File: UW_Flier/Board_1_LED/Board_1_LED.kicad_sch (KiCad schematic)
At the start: 11 parts, among them J1 RESET, J2 SWDIO, J3 SWDCLK, J4 GND, J5 VDD, J6 LED_DRAIN, Q1 CSD13385F5, U1 EYSHSNZWZ_module_stub

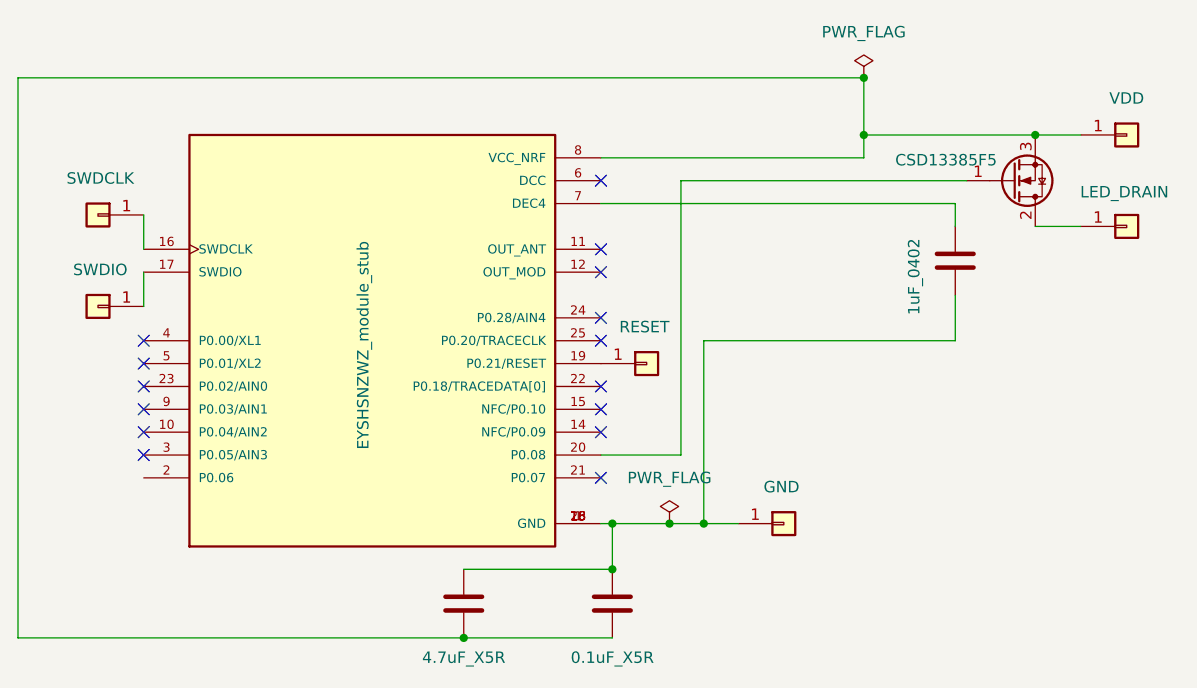
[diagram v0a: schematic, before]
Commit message: stuff
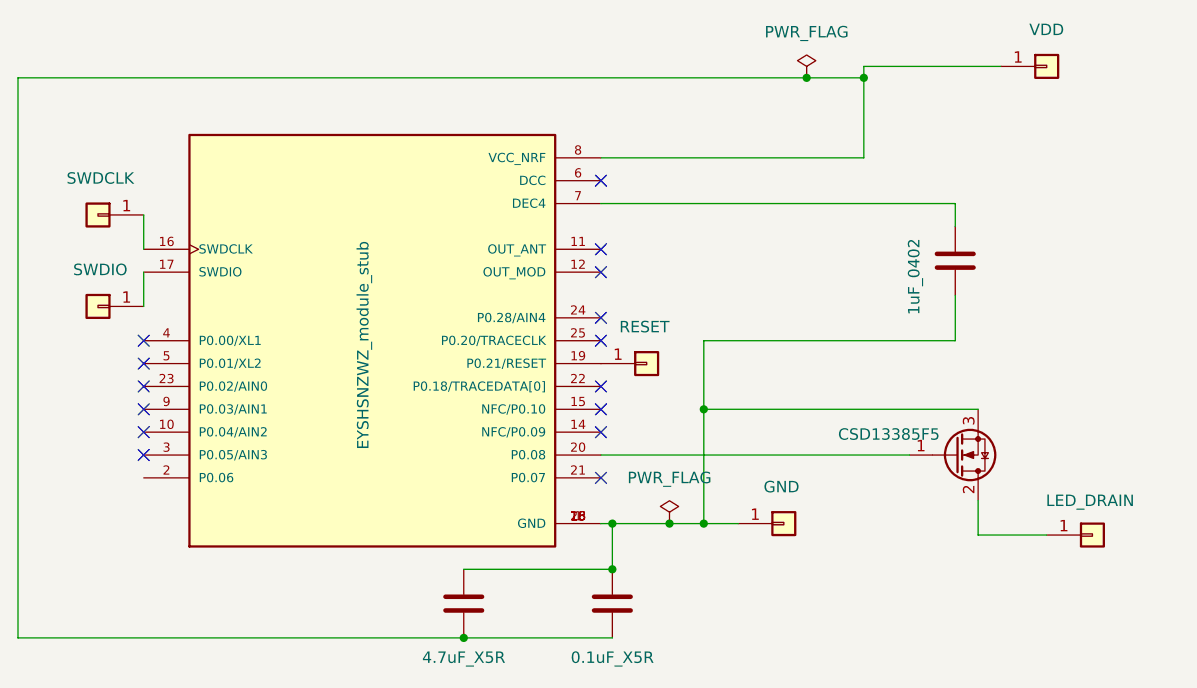
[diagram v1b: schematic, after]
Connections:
- net at C1.2, C2.2, C3.2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: now also Q1.3 (S)
- net at C1.1, C2.1, J5.1 (Pin_1)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: no longer Q1.3 (S)
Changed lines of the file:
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@@
+	)
+	(junction
+		(at 119.38 43.18)
+		(diameter 0)
+		(color 0 0 0 0)
 	)
 	(junction
@@
 	)
 	(junction
-		(at 144.78 49.53)
-		(diameter 0)
-		(color 0 0 0 0)
-	)
-	(junction
 		(at 107.95 92.71)
-		(diameter 0)
-		(color 0 0 0 0)
-	)
-	(junction
-		(at 125.73 49.53)
 		(diameter 0)
 		(color 0 0 0 0)
@@
 	)
 	(junction
+		(at 107.95 80.01)
+		(diameter 0)
+		(color 0 0 0 0)
+	)
+	(junction
 		(at 97.79 97.79)
 		(diameter 0)
@@
 	(wire
 		(pts
-			(xy 125.73 43.18) (xy 125.73 49.53)
+			(xy 125.73 43.18) (xy 125.73 52.07)
 		)
 		(stroke
@@
 	(wire
 		(pts
+			(xy 140.97 41.91) (xy 125.73 41.91)
+		)
+		(stroke
+			(width 0)
+			(type default)
+		)
+	)
+	(wire
+		(pts
 			(xy 31.75 105.41) (xy 31.75 43.18)
 		)
@@
 	(wire
 		(pts
-			(xy 144.78 59.69) (xy 149.86 59.69)
-		)
-		(stroke
-			(width 0)
-			(type default)
-		)
-	)
-	(wire
-		(pts
 			(xy 135.89 67.31) (xy 135.89 72.39)
 		)
@@
 	(wire
 		(pts
+			(xy 125.73 41.91) (xy 125.73 43.18)
+		)
+		(stroke
+			(width 0)
+			(type default)
+		)
+	)
+	(wire
+		(pts
 			(xy 97.79 92.71) (xy 104.14 92.71)
 		)
@@
 	(wire
 		(pts
-			(xy 125.73 49.53) (xy 144.78 49.53)
+			(xy 138.43 93.98) (xy 138.43 90.17)
+		)
+		(stroke
+			(width 0)
+			(type default)
+		)
+	)
+	(wire
+		(pts
+			(xy 107.95 80.01) (xy 138.43 80.01)
+		)
+		(stroke
+			(width 0)
+			(type default)
+		)
+	)
+	(wire
+		(pts
+			(xy 107.95 80.01) (xy 107.95 92.71)
 		)
 		(stroke
@@
 	(wire
 		(pts
-			(xy 144.78 49.53) (xy 149.86 49.53)
-		)
-		(stroke
-			(width 0)
-			(type default)
-		)
-	)
-	(wire
-		(pts
 			(xy 96.52 52.07) (xy 125.73 52.07)
 		)
@@
 	(wire
 		(pts
+			(xy 146.05 93.98) (xy 138.43 93.98)
+		)
+		(stroke
+			(width 0)
+			(type default)
+		)
+	)
+	(wire
+		(pts
+			(xy 119.38 43.18) (xy 125.73 43.18)
+		)
+		(stroke
+			(width 0)
+			(type default)
+		)
+	)
+	(wire
+		(pts
 			(xy 97.79 92.71) (xy 97.79 97.79)
 		)
@@
 	(wire
 		(pts
-			(xy 107.95 72.39) (xy 107.95 92.71)
+			(xy 107.95 72.39) (xy 107.95 80.01)
 		)
 		(stroke
@@
 	(wire
 		(pts
-			(xy 96.52 85.09) (xy 105.41 85.09)
+			(xy 96.52 85.09) (xy 130.81 85.09)
 		)
 		(stroke
@@
 	(wire
 		(pts
-			(xy 31.75 43.18) (xy 125.73 43.18)
-		)
-		(stroke
-			(width 0)
-			(type default)
-		)
-	)
-	(wire
-		(pts
-			(xy 105.41 54.61) (xy 137.16 54.61)
+			(xy 31.75 43.18) (xy 119.38 43.18)
 		)
 		(stroke
@@
 		(pts
 			(xy 135.89 57.15) (xy 135.89 59.69)
-		)
-		(stroke
-			(width 0)
-			(type default)
-		)
-	)
-	(wire
-		(pts
-			(xy 125.73 52.07) (xy 125.73 49.53)
-		)
-		(stroke
-			(width 0)
-			(type default)
-		)
-	)
-	(wire
-		(pts
-			(xy 105.41 54.61) (xy 105.41 85.09)
 		)
 		(stroke
@@
 	(symbol
 		(lib_id "power:PWR_FLAG")
-		(at 125.73 43.18 0)
+		(at 119.38 43.18 0)
 		(unit 1)
 		(exclude_from_sim no)
@@
 		(fields_autoplaced yes)
 		(property "Reference" "#FLG01"
-			(at 125.73 41.275 0)
+			(at 119.38 41.275 0)
 			(effects
 				(font
@@
 		)
 		(property "Value" "PWR_FLAG"
-			(at 125.73 38.1 0)
+			(at 119.38 38.1 0)
 			(effects
 				(font
@@
 		)
 		(property "Footprint" ""
-			(at 125.73 43.18 0)
+			(at 119.38 43.18 0)
 			(effects
 				(font
@@
 		)
 		(property "Datasheet" "~"
-			(at 125.73 43.18 0)
+			(at 119.38 43.18 0)
 			(effects
 				(font
@@
 		)
 		(property "Description" "Special symbol for telling ERC where power comes from"
-			(at 125.73 43.18 0)
+			(at 119.38 43.18 0)
 			(effects
 				(font
@@
 	(symbol
 		(lib_id "Connector_Generic:Conn_01x01")
-		(at 154.94 49.53 0)
+		(at 146.05 41.91 0)
 		(unit 1)
 		(exclude_from_sim no)
@@
 		(dnp no)
 		(property "Reference" "J5"
-			(at 154.94 46.53 0)
+			(at 146.05 38.91 0)
 			(effects
 				(font
@@
 		)
 		(property "Value" "VDD"
-			(at 154.94 45.466 0)
+			(at 146.05 37.846 0)
 			(effects
 				(font
@@
 		)
 		(property "Footprint" "TestPoint:TestPoint_Pad_2.0x2.0mm"
-			(at 154.94 49.53 0)
+			(at 146.05 41.91 0)
 			(effects
 				(font
@@
 		)
 		(property "Datasheet" "~"
-			(at 154.94 49.53 0)
+			(at 146.05 41.91 0)
 			(effects
 				(font
@@
 		)
 		(property "Description" "Generic connector, single row, 01x01, script generated (kicad-library-utils/schlib/autogen/connector/)"
-			(at 154.94 49.53 0)
+			(at 146.05 41.91 0)
 			(effects
 				(font
@@
 	(symbol
 		(lib_id "Connector_Generic:Conn_01x01")
-		(at 154.94 59.69 0)
+		(at 151.13 93.98 0)
 		(unit 1)
 		(exclude_from_sim no)
@@
 		(dnp no)
 		(property "Reference" "J6"
-			(at 154.94 56.69 0)
+			(at 151.13 90.98 0)
 			(effects
 				(font
@@
 		)
 		(property "Value" "LED_DRAIN"
-			(at 154.686 55.88 0)
+			(at 150.876 90.17 0)
 			(effects
 				(font
@@
 		)
 		(property "Footprint" "TestPoint:TestPoint_Pad_2.0x2.0mm"
-			(at 154.94 59.69 0)
+			(at 151.13 93.98 0)
 			(effects
 				(font
@@
 		)
 		(property "Datasheet" "~"
-			(at 154.94 59.69 0)
+			(at 151.13 93.98 0)
 			(effects
 				(font
@@
 		)
 		(property "Description" "Generic connector, single row, 01x01, script generated (kicad-library-utils/schlib/autogen/connector/)"
-			(at 154.94 59.69 0)
+			(at 151.13 93.98 0)
 			(effects
 				(font
@@
 	(symbol
 		(lib_id "Transistor_FET:Q_NMOS_GDS")
-		(at 142.24 54.61 0)
+		(at 135.89 85.09 0)
 		(mirror x)
 		(unit 1)
@@
 		(dnp no)
 		(property "Reference" "Q1"
-			(at 142.24 58.61 0)
+			(at 135.89 89.09 0)
 			(effects
 				(font
@@
 		)
 		(property "Value" "CSD13385F5"
-			(at 134.874 52.324 0)
+			(at 128.524 82.804 0)
 			(effects
 				(font
@@
 		)
 		(property "Footprint" "CSD13385F5:TRANS_CSD13385F5"
-			(at 147.32 57.15 0)
+			(at 140.97 87.63 0)
 			(effects
 				(font
@@
 		)
 		(property "Datasheet" "~"
-			(at 142.24 54.61 0)
+			(at 135.89 85.09 0)
 			(effects
 				(font
@@
 		)
 		(property "Description" "N-MOSFET transistor, gate/drain/source"
-			(at 142.24 54.61 0)
-			(effects
-				(font
+			(at 135.89 85.09 0)
+			(effects
+				(font

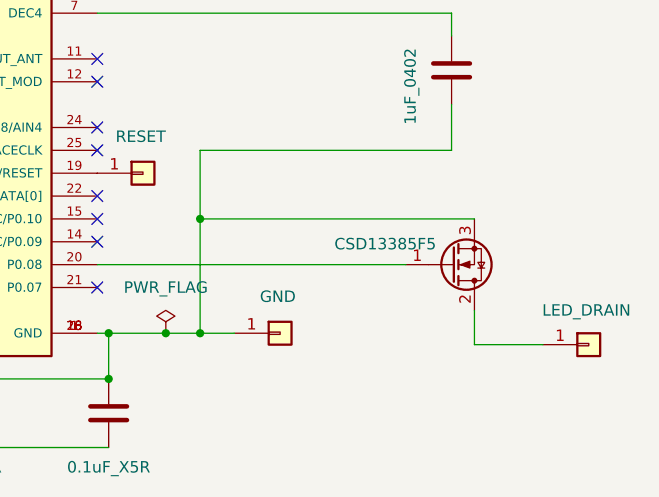
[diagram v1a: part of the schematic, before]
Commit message: updated PCB
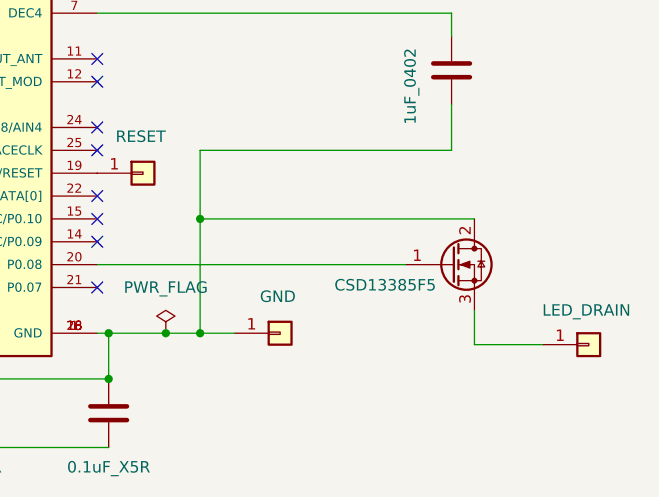
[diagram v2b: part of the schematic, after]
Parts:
- C1: footprint Capacitor_SMD:C_0603_1608Metric -> Capacitor_SMD:C_0402_1005Metric
- J1, J2, J3, J4, J5, J6: footprint TestPoint:TestPoint_Pad_2.0x2.0mm -> CSD13385F5:TestPoint_Pad_1.5x1.5mm_2
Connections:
- net at C1.2, C2.2, C3.2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: now also Q1.2 (D); no longer Q1.3 (S)
- net at J6.1 (Pin_1): now also Q1.3 (S); no longer Q1.2 (D)
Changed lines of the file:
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@@
+	)
+	(junction
+		(at 107.95 80.01)
+		(diameter 0)
+		(color 0 0 0 0)
 	)
 	(junction
@@
 	)
 	(junction
-		(at 107.95 80.01)
-		(diameter 0)
-		(color 0 0 0 0)
-	)
-	(junction
 		(at 97.79 97.79)
 		(diameter 0)
@@
 	(wire
 		(pts
+			(xy 138.43 90.17) (xy 138.43 93.98)
+		)
+		(stroke
+			(width 0)
+			(type default)
+		)
+	)
+	(wire
+		(pts
 			(xy 140.97 41.91) (xy 125.73 41.91)
 		)
@@
 	(wire
 		(pts
-			(xy 138.43 93.98) (xy 138.43 90.17)
+			(xy 107.95 72.39) (xy 107.95 80.01)
+		)
+		(stroke
+			(width 0)
+			(type default)
+		)
+	)
+	(wire
+		(pts
+			(xy 45.72 58.42) (xy 45.72 62.23)
+		)
+		(stroke
+			(width 0)
+			(type default)
+		)
+	)
+	(wire
+		(pts
+			(xy 135.89 72.39) (xy 107.95 72.39)
+		)
+		(stroke
+			(width 0)
+			(type default)
+		)
+	)
+	(wire
+		(pts
+			(xy 96.52 57.15) (xy 135.89 57.15)
 		)
 		(stroke
@@
 	(wire
 		(pts
-			(xy 45.72 58.42) (xy 45.72 62.23)
-		)
-		(stroke
-			(width 0)
-			(type default)
-		)
-	)
-	(wire
-		(pts
-			(xy 135.89 72.39) (xy 107.95 72.39)
-		)
-		(stroke
-			(width 0)
-			(type default)
-		)
-	)
-	(wire
-		(pts
-			(xy 96.52 57.15) (xy 135.89 57.15)
-		)
-		(stroke
-			(width 0)
-			(type default)
-		)
-	)
-	(wire
-		(pts
 			(xy 96.52 52.07) (xy 125.73 52.07)
 		)
@@
 		(pts
 			(xy 97.79 92.71) (xy 97.79 97.79)
-		)
-		(stroke
-			(width 0)
-			(type default)
-		)
-	)
-	(wire
-		(pts
-			(xy 107.95 72.39) (xy 107.95 80.01)
 		)
 		(stroke
@@
 			)
 		)
-		(property "Footprint" "TestPoint:TestPoint_Pad_2.0x2.0mm"
+		(property "Footprint" "CSD13385F5:TestPoint_Pad_1.5x1.5mm_2"
 			(at 40.64 58.42 0)
 			(effects
@@
 			)
 		)
-		(property "Footprint" "TestPoint:TestPoint_Pad_2.0x2.0mm"
+		(property "Footprint" "CSD13385F5:TestPoint_Pad_1.5x1.5mm_2"
 			(at 146.05 41.91 0)
 			(effects
@@
 			)
 		)
-		(property "Footprint" "TestPoint:TestPoint_Pad_2.0x2.0mm"
+		(property "Footprint" "CSD13385F5:TestPoint_Pad_1.5x1.5mm_2"
 			(at 116.84 92.71 0)
 			(effects
@@
 			)
 		)
-		(property "Footprint" "Capacitor_SMD:C_0603_1608Metric"
+		(property "Footprint" "Capacitor_SMD:C_0402_1005Metric"
 			(at 82.2452 97.79 0)
 			(effects
@@
 			)
 		)
-		(property "Footprint" "TestPoint:TestPoint_Pad_2.0x2.0mm"
+		(property "Footprint" "CSD13385F5:TestPoint_Pad_1.5x1.5mm_2"
 			(at 101.6 74.93 0)
 			(effects
@@
 			)
 		)
-		(property "Footprint" "TestPoint:TestPoint_Pad_2.0x2.0mm"
+		(property "Footprint" "CSD13385F5:TestPoint_Pad_1.5x1.5mm_2"
 			(at 40.64 68.58 0)
 			(effects
@@
 			)
 		)
-		(property "Footprint" "TestPoint:TestPoint_Pad_2.0x2.0mm"
+		(property "Footprint" "CSD13385F5:TestPoint_Pad_1.5x1.5mm_2"
 			(at 151.13 93.98 0)
 			(effects
@@
 		(lib_id "Transistor_FET:Q_NMOS_GDS")
 		(at 135.89 85.09 0)
-		(mirror x)
 		(unit 1)
 		(exclude_from_sim no)
@@
 		(dnp no)
 		(property "Reference" "Q1"
-			(at 135.89 89.09 0)
+			(at 135.89 81.09 0)
 			(effects
 				(font
@@
 		)
 		(property "Value" "CSD13385F5"
-			(at 128.524 82.804 0)
+			(at 128.524 87.376 0)
 			(effects
 				(font
@@
 		)
 		(property "Footprint" "CSD13385F5:TRANS_CSD13385F5"
-			(at 140.97 87.63 0)
-			(effects
-				(font
+			(at 140.97 82.55 0)
+			(effects
+				(font

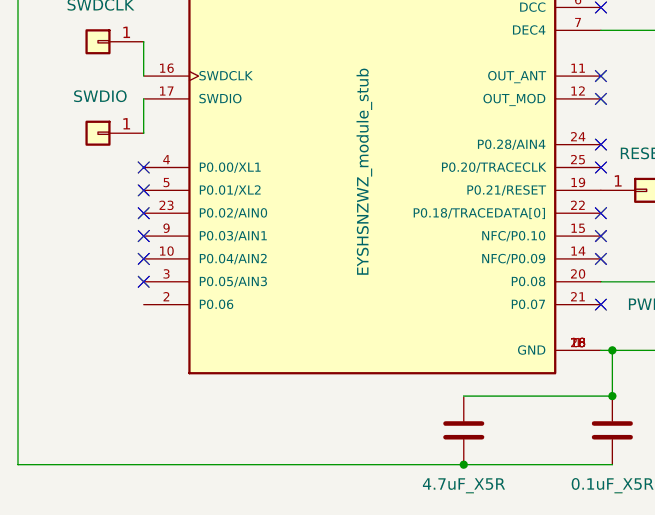
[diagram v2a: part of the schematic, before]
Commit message: stuff (thursday before leaving)
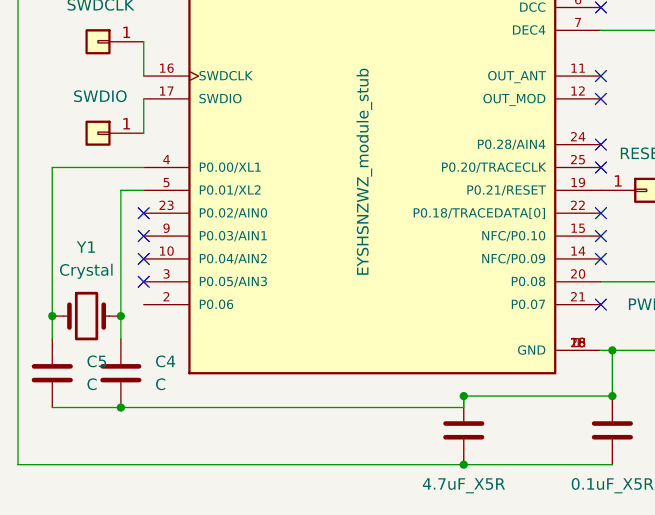
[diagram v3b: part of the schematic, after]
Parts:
- added C4, C5: C, Capacitor_SMD:C_0201_0603Metric_Pad0.64x0.40mm_HandSolder, symbol Device:C
- added Y1: Crystal, Capacitor_SMD:C_0402_1005Metric, symbol Device:Crystal
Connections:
- net at C1.2, C2.2, C3.2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: now also C4.2, C5.2
- net at U1.4 (P0.00/XL1): now also C5.1, Y1.1
- net at U1.5 (P0.01/XL2): now also C4.1, Y1.2
- no-connect marks 15 -> 13
